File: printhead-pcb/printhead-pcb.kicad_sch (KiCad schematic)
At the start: 30 parts, among them J1 Power, J2 DSCL, J3 DSDA, U1 PCA9615DP, U6 AP7361C-33E

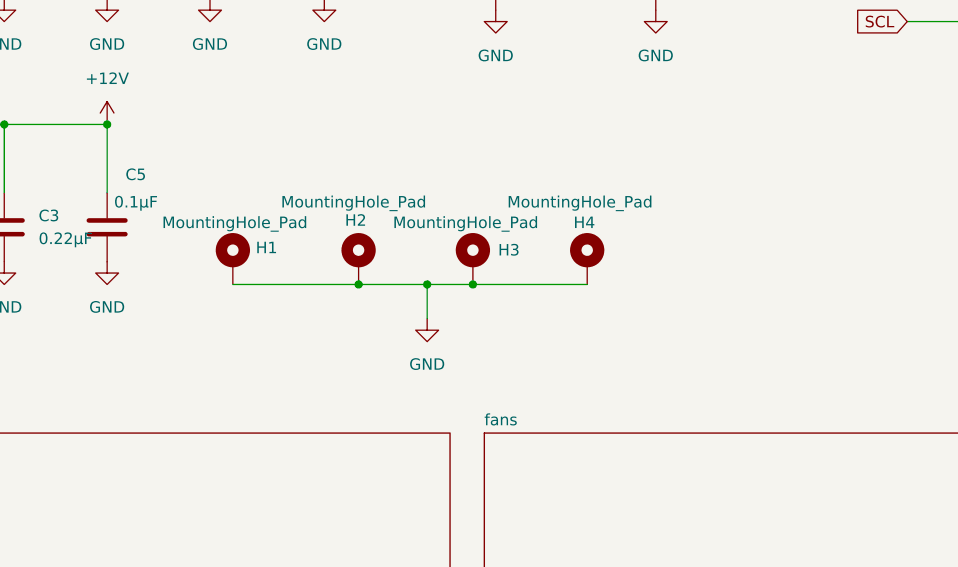
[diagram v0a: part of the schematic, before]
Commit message: created pi pcb and added ToDo Doc
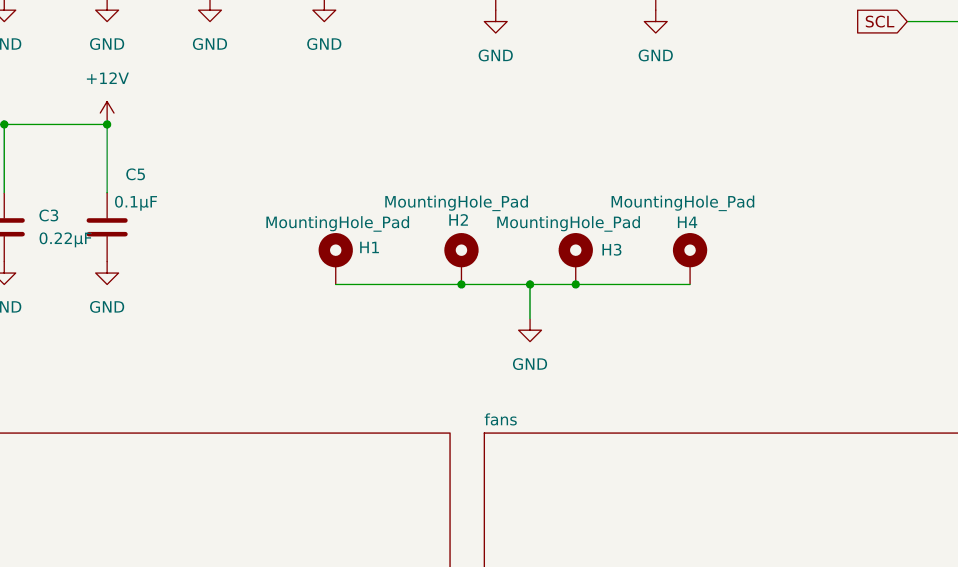
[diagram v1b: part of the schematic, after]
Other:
- moved on the sheet: H1, H2, H3, H4
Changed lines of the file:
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@@
 	)
 	(junction
-		(at 113.03 72.39)
+		(at 124.46 72.39)
 		(diameter 0)
 		(color 0 0 0 0)
 	)
 	(junction
-		(at 107.95 72.39)
+		(at 119.38 72.39)
 		(diameter 0)
 		(color 0 0 0 0)
@@
 	)
 	(junction
-		(at 100.33 72.39)
+		(at 111.76 72.39)
 		(diameter 0)
 		(color 0 0 0 0)
@@
 	(wire
 		(pts
-			(xy 86.36 72.39) (xy 100.33 72.39)
+			(xy 97.79 72.39) (xy 111.76 72.39)
 		)
 		(stroke
@@
 	(wire
 		(pts
-			(xy 107.95 72.39) (xy 107.95 76.2)
+			(xy 119.38 72.39) (xy 119.38 76.2)
 		)
 		(stroke
@@
 	(wire
 		(pts
-			(xy 113.03 72.39) (xy 125.73 72.39)
+			(xy 124.46 72.39) (xy 137.16 72.39)
 		)
 		(stroke
@@
 	(wire
 		(pts
-			(xy 107.95 72.39) (xy 113.03 72.39)
+			(xy 119.38 72.39) (xy 124.46 72.39)
 		)
 		(stroke
@@
 	(wire
 		(pts
-			(xy 100.33 72.39) (xy 107.95 72.39)
+			(xy 111.76 72.39) (xy 119.38 72.39)
 		)
 		(stroke
@@
 		(lib_name "MountingHole_Pad_2")
 		(lib_id "Mechanical:MountingHole_Pad")
-		(at 113.03 69.85 0)
+		(at 124.46 69.85 0)
 		(unit 1)
 		(exclude_from_sim no)
@@
 		(dnp no)
 		(property "Reference" "H3"
-			(at 115.824 68.58 0)
+			(at 127.254 68.58 0)
 			(effects
 				(font
@@
 		)
 		(property "Value" "MountingHole_Pad"
-			(at 104.14 65.532 0)
+			(at 115.57 65.532 0)
 			(effects
 				(font
@@
 		)
 		(property "Footprint" "MountingHole:MountingHole_2.2mm_M2_Pad_TopBottom"
-			(at 113.03 69.85 0)
+			(at 124.46 69.85 0)
 			(effects
 				(font
@@
 		)
 		(property "Datasheet" "~"
-			(at 113.03 69.85 0)
+			(at 124.46 69.85 0)
 			(effects
 				(font
@@
 		)
 		(property "Description" "Mounting Hole with connection"
-			(at 113.03 69.85 0)
+			(at 124.46 69.85 0)
 			(effects
 				(font
@@
 		(lib_name "MountingHole_Pad_1")
 		(lib_id "Mechanical:MountingHole_Pad")
-		(at 125.73 69.85 0)
+		(at 137.16 69.85 0)
 		(unit 1)
 		(exclude_from_sim no)
@@
 		(dnp no)
 		(property "Reference" "H4"
-			(at 124.206 65.532 0)
+			(at 135.636 65.532 0)
 			(effects
 				(font
@@
 		)
 		(property "Value" "MountingHole_Pad"
-			(at 116.84 63.246 0)
+			(at 128.27 63.246 0)
 			(effects
 				(font
@@
 		)
 		(property "Footprint" "MountingHole:MountingHole_2.2mm_M2_Pad_TopBottom"
-			(at 125.73 69.85 0)
+			(at 137.16 69.85 0)
 			(effects
 				(font
@@
 		)
 		(property "Datasheet" "~"
-			(at 125.73 69.85 0)
+			(at 137.16 69.85 0)
 			(effects
 				(font
@@
 		)
 		(property "Description" "Mounting Hole with connection"
-			(at 125.73 69.85 0)
+			(at 137.16 69.85 0)
 			(effects
 				(font
@@
 	(symbol
 		(lib_id "power:GND")
-		(at 107.95 76.2 0)
+		(at 119.38 76.2 0)
 		(unit 1)
 		(exclude_from_sim no)
@@
 		(fields_autoplaced yes)
 		(property "Reference" "#PWR012"
-			(at 107.95 82.55 0)
+			(at 119.38 82.55 0)
 			(effects
 				(font
@@
 		)
 		(property "Value" "GND"
-			(at 107.95 81.28 0)
+			(at 119.38 81.28 0)
 			(effects
 				(font
@@
 		)
 		(property "Footprint" ""
-			(at 107.95 76.2 0)
+			(at 119.38 76.2 0)
 			(effects
 				(font
@@
 		)
 		(property "Datasheet" ""
-			(at 107.95 76.2 0)
+			(at 119.38 76.2 0)
 			(effects
 				(font
@@
 		)
 		(property "Description" "Power symbol creates a global label with name \"GND\" , ground"
-			(at 107.95 76.2 0)
+			(at 119.38 76.2 0)
 			(effects
 				(font
@@
 		(lib_name "MountingHole_Pad_3")
 		(lib_id "Mechanical:MountingHole_Pad")
-		(at 100.33 69.85 0)
+		(at 111.76 69.85 0)
 		(unit 1)
 		(exclude_from_sim no)
@@
 		(dnp no)
 		(property "Reference" "H2"
-			(at 98.806 65.278 0)
+			(at 110.236 65.278 0)
 			(effects
 				(font
@@
 		)
 		(property "Value" "MountingHole_Pad"
-			(at 91.694 63.246 0)
+			(at 103.124 63.246 0)
 			(effects
 				(font
@@
 		)
 		(property "Footprint" "MountingHole:MountingHole_2.2mm_M2_Pad_TopBottom"
-			(at 100.33 69.85 0)
+			(at 111.76 69.85 0)
 			(effects
 				(font
@@
 		)
 		(property "Datasheet" "~"
-			(at 100.33 69.85 0)
+			(at 111.76 69.85 0)
 			(effects
 				(font
@@
 		)
 		(property "Description" "Mounting Hole with connection"
-			(at 100.33 69.85 0)
+			(at 111.76 69.85 0)
 			(effects
 				(font
@@
 	(symbol
 		(lib_id "Mechanical:MountingHole_Pad")
-		(at 86.36 69.85 0)
+		(at 97.79 69.85 0)
 		(unit 1)
 		(exclude_from_sim no)
@@
 		(dnp no)
 		(property "Reference" "H1"
-			(at 88.9 68.326 0)
+			(at 100.33 68.326 0)
 			(effects
 				(font
@@
 		)
 		(property "Value" "MountingHole_Pad"
-			(at 78.486 65.532 0)
+			(at 89.916 65.532 0)
 			(effects
 				(font
@@
 		)
 		(property "Footprint" "MountingHole:MountingHole_2.2mm_M2_Pad_TopBottom"
-			(at 86.36 69.85 0)
+			(at 97.79 69.85 0)
 			(effects
 				(font
@@
 		)
 		(property "Datasheet" "~"
-			(at 86.36 69.85 0)
+			(at 97.79 69.85 0)
 			(effects
 				(font
@@
 		)
 		(property "Description" "Mounting Hole with connection"
-			(at 86.36 69.85 0)
+			(at 97.79 69.85 0)
 			(effects
 				(font
